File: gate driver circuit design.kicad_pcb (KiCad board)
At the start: 2 copper layers, 40 x 40 mm, 105 parts, among them J101 90122-0763, J102 90121-0762, J103 90121-0762, Q1 CSD17313Q2, Q2 MMBT3904T-7-F, Q3 MMBT3904T-7-F, Q4 MMBT3904T-7-F, T1 750343725, T2 750343725, U1 SN6501QDBVRQ1, U2 TPS7B6950QDCYRQ1, U3 TL431AQDBZRQ1, U4 SN6501QDBVRQ1, U5 TL431AQDBZRQ1, U6 UCC21530QDWKRQ1, U7 ISO7721QDRQ1, U8 LMV762QMA_NOPB, U9 TL431AQDBZRQ1

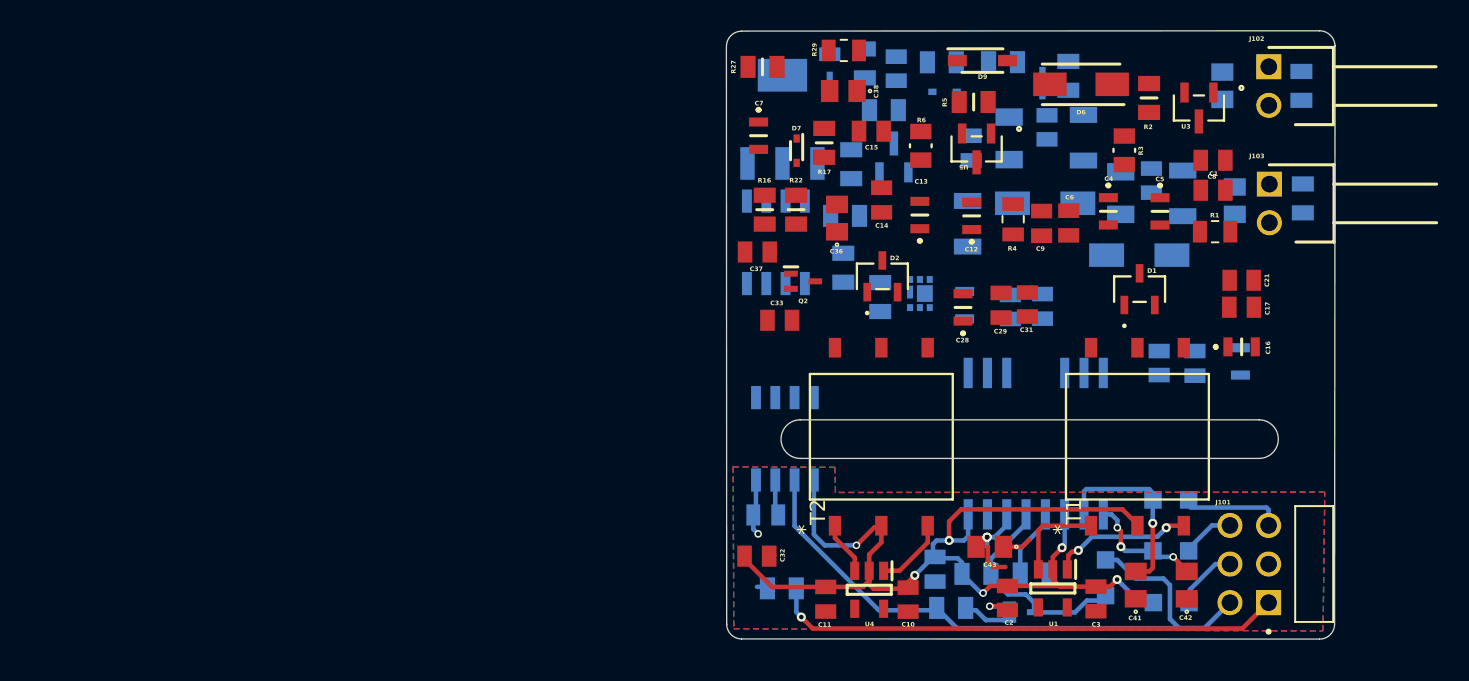
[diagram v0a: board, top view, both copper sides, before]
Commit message: PCB Routing Last Stage
PCB Routing Last Stage
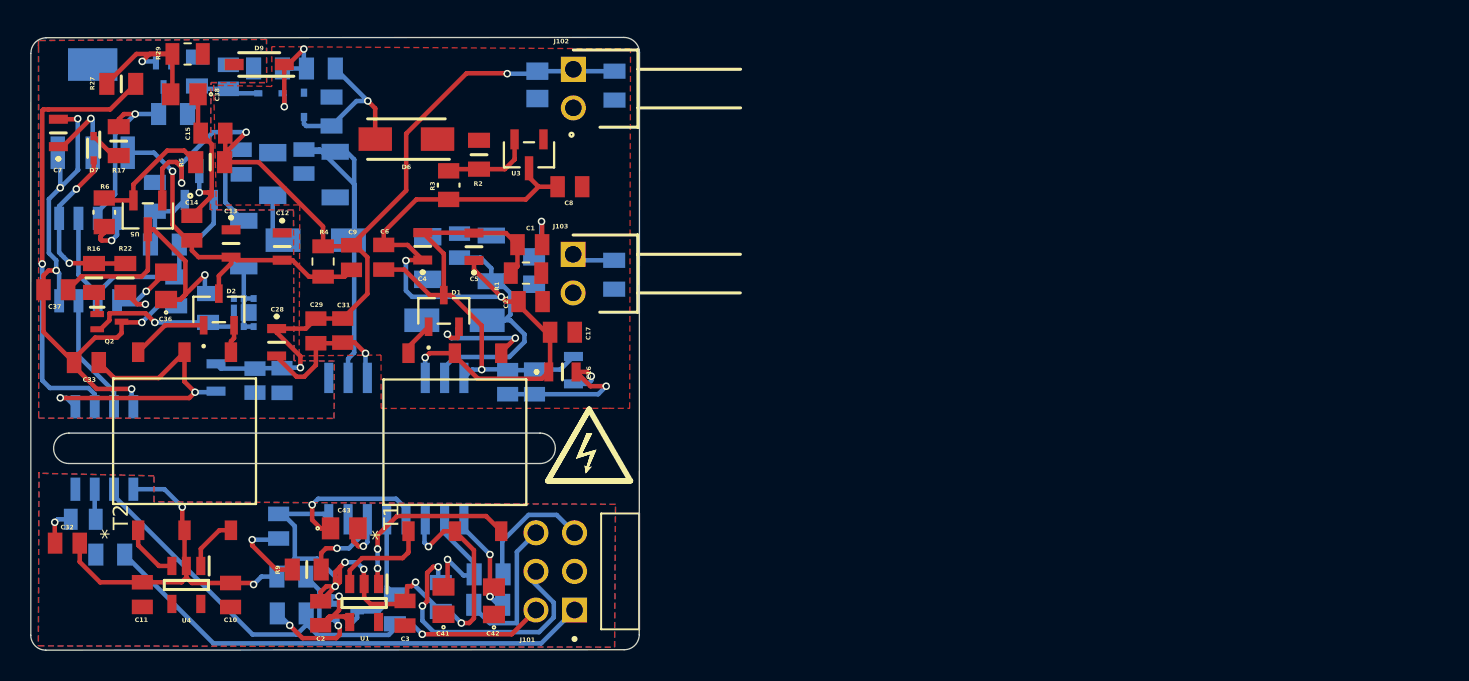
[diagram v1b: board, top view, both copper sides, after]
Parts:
- R132, R31, R33, R34: footprint ERJ-U060R00V:ERJS06_U06__0805_ -> CR0805-FX-5101ELF:RESC2012X60N
- R9: moved to F.Cu
- moved U5 54.7 mm to (39.9, 59.0)
- moved R6 53.9 mm to (37.0, 58.8)
- moved R5 50.4 mm to (44.0, 55.5)
- moved C27 50.3 mm to (48.7, 69.9)
- moved C30 49.9 mm to (46.9, 69.9)
- moved C26 49.5 mm to (44.4, 69.7)
- moved R10 49.3 mm to (52.2, 56.3)
- moved C24 48.9 mm to (50.2, 55.5)
- moved D5 48.6 mm to (50.2, 51.7)
- moved R15 48.5 mm to (52.0, 52.2)
- moved R11 48.5 mm to (48.1, 56.3), turned to 90 degrees
- moved R132 48.0 mm to (59.2, 84.1), turned to -90 degrees
- moved D4 48.0 mm to (50.9, 60.6)
- moved C25 48.0 mm to (46.0, 55.5)
- moved R9 47.9 mm to (50.3, 82.3), turned to 0 degrees
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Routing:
- net Comb: track 0.00 -> 71.0 mm, vias 0 -> 4
- net -4Vb: track 0.00 -> 60.1 mm, vias 0 -> 6
- net -4Va: track 0.00 -> 48.2 mm, vias 0 -> 3
- net Vcc5V: track 0.00 -> 39.0 mm, vias 0 -> 5
- net +15Vb: track 0.00 -> 33.6 mm, vias 0 -> 2
- net +15Va: track 0.00 -> 32.0 mm, vias 0 -> 1
- net Net-(U7-OUTB): track 0.00 -> 29.3 mm, vias 0 -> 1
- net Net-(D4-K): track 0.00 -> 26.2 mm
- net Net-(U8--IN_A): track 0.00 -> 18.7 mm
- net Coma: track 0.00 -> 18.7 mm, vias 0 -> 3
- net Net-(D3-K): track 0.00 -> 17.9 mm
- net Net-(J101-Pad4): track 4.59 -> 18.5 mm, vias 0 -> 2
- net Net-(Q3-C): track 0.00 -> 13.0 mm, vias 0 -> 1
- net Net-(D7-A): track 0.00 -> 11.7 mm, vias 0 -> 2
- net Net-(D5-A): track 0.00 -> 11.1 mm, vias 0 -> 1
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- added copper zone on B.Cu, net -4Vb
- added copper zone on F.Cu, net -4Vb
- added copper zone on F.Cu, net Coma
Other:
- board size 40 x 40 mm -> 40 x 40.3 mm
